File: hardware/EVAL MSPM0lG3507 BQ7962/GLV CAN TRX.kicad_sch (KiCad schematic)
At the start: 29 parts, among them U10 MCP2542FDxMF, U11 FCX495, U8 FCX495, U9 LMR51603XDBVR

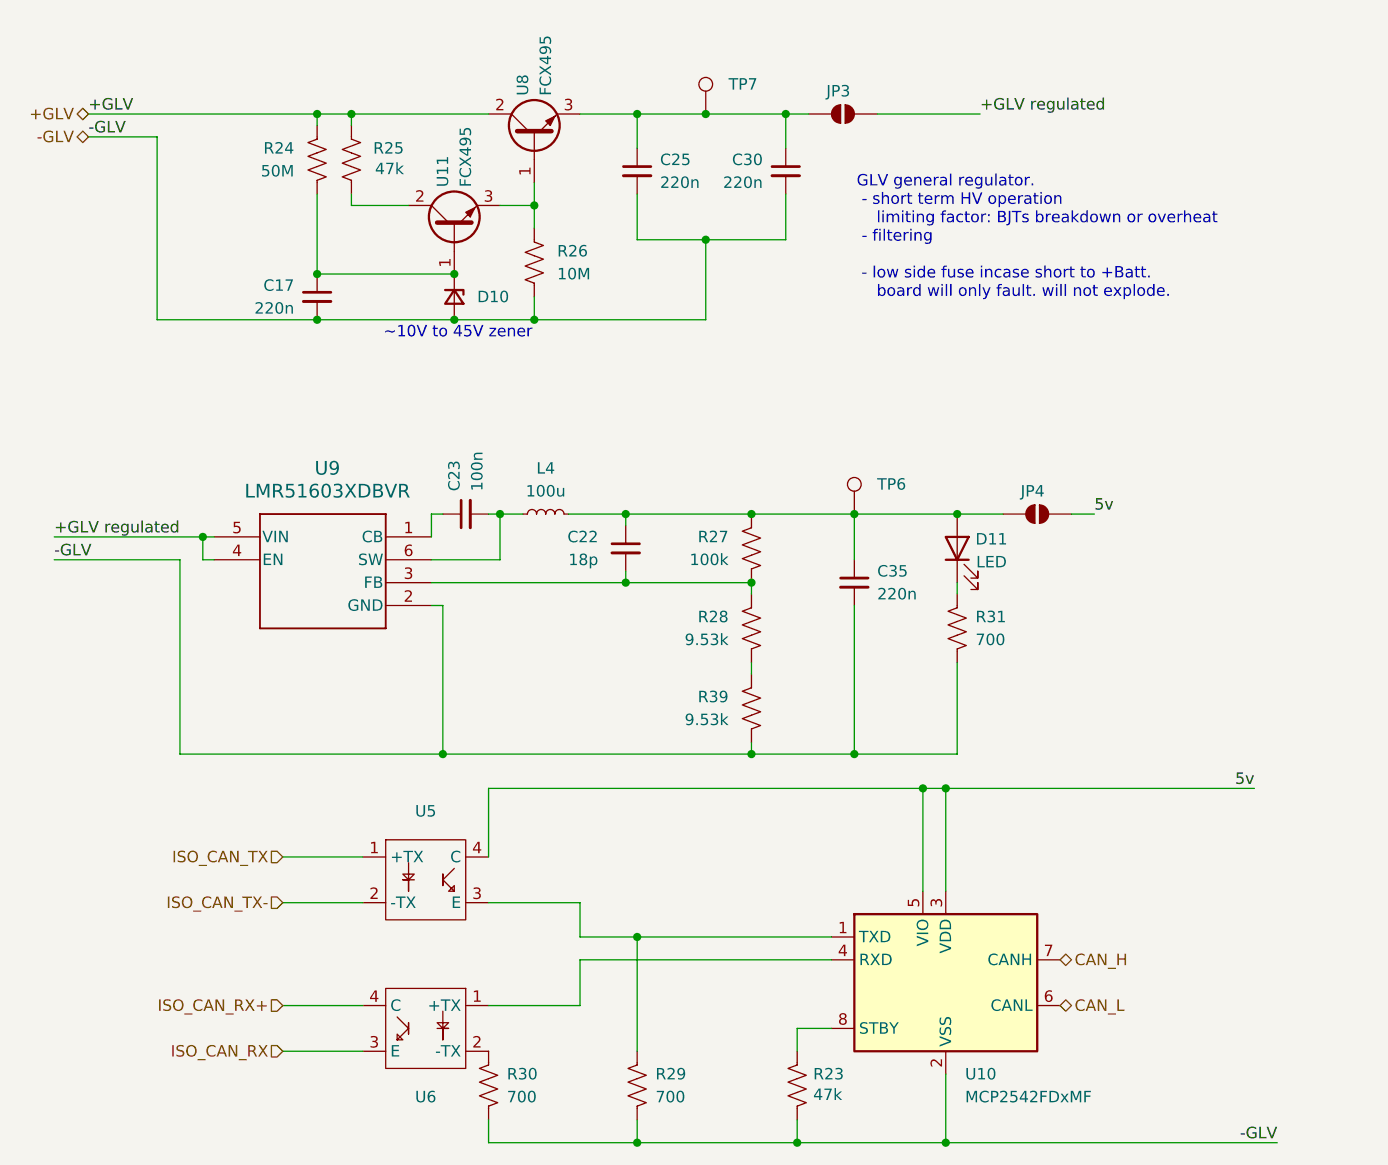
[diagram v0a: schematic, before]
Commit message: cleaned up schematics
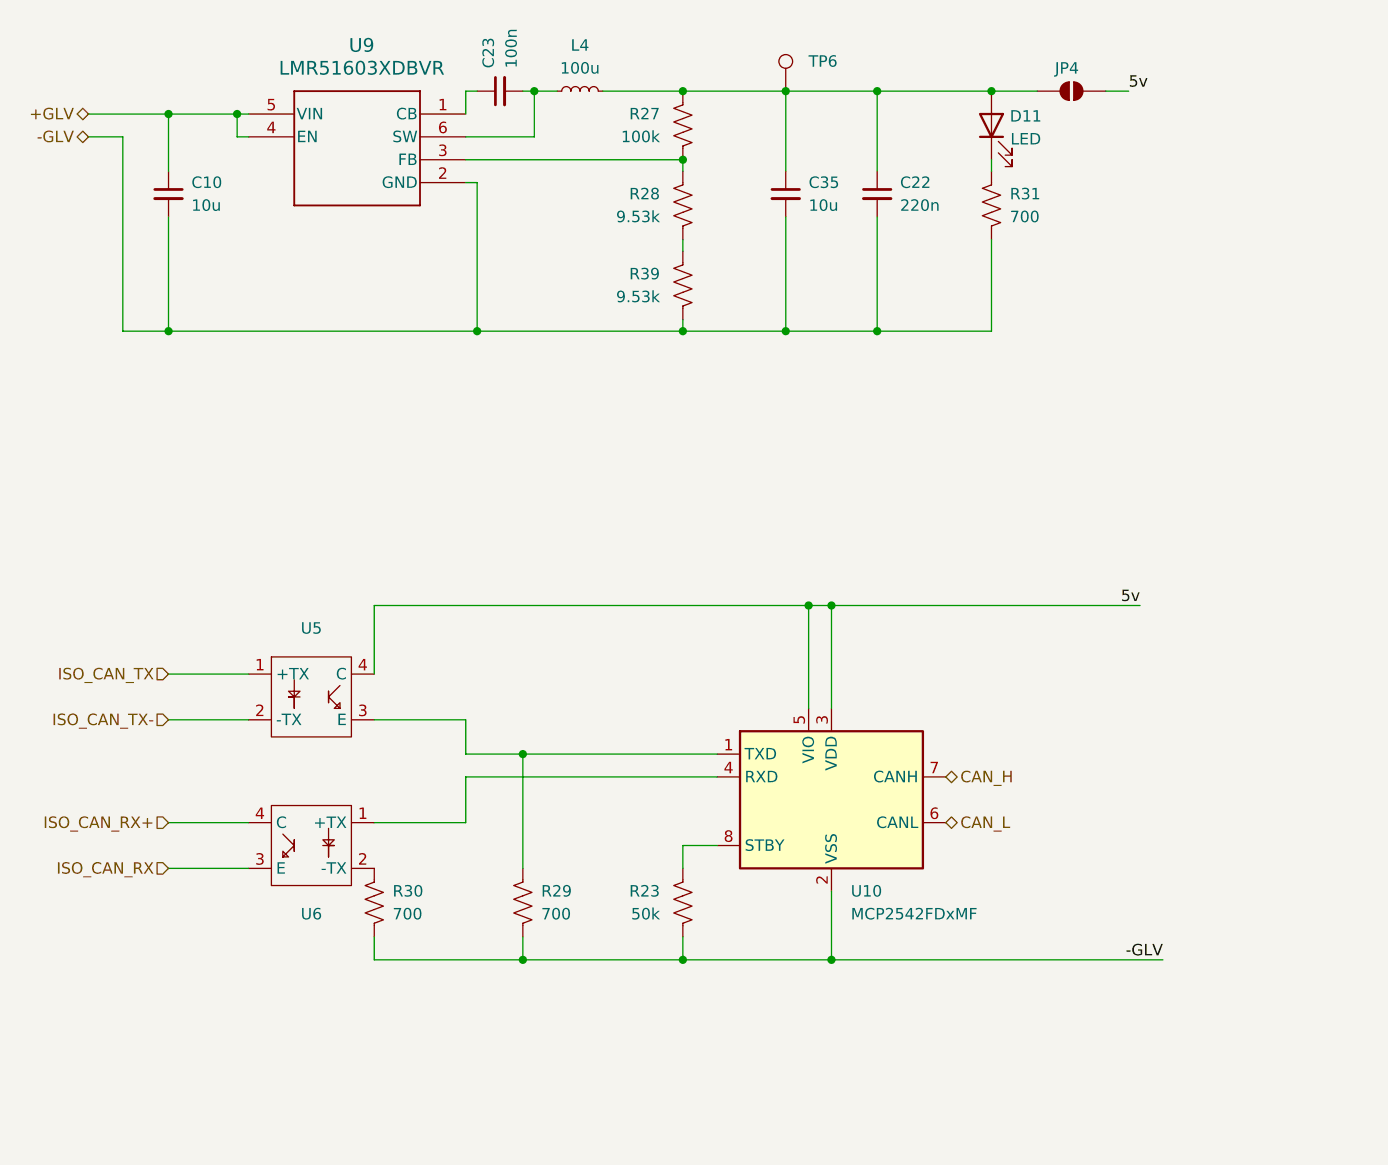
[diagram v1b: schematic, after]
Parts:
- removed C17, C25, C30: 220n, Capacitor_SMD:C_1206_3216Metric_Pad1.33x1.80mm_HandSolder, symbol Device:C_Small
- removed D10: 36V, Diode_SMD:D_SOD-123, symbol Device:D_Zener_Small
- removed JP3: SolderJumper_2_Open, Jumper:SolderJumper-2_P1.3mm_Open_TrianglePad1.0x1.5mm, symbol Jumper:SolderJumper_2_Open
- removed R24: 50M, Resistor_SMD:R_1206_3216Metric_Pad1.30x1.75mm_HandSolder, symbol Device:R_US
- removed R25: 47k, Resistor_SMD:R_1206_3216Metric_Pad1.30x1.75mm_HandSolder, symbol Device:R_US
- removed R26: 10M, Resistor_SMD:R_1206_3216Metric_Pad1.30x1.75mm_HandSolder, symbol Device:R_US
- removed TP7: TestPoint, TestPoint:TestPoint_Loop_D2.50mm_Drill1.0mm_LowProfile, symbol Connector:TestPoint
- removed U11, U8: FCX495, Package_TO_SOT_SMD:SOT-89-3, symbol zzLocalLibrary:FCX485_NPN_BJT
- added C10: 10u, Capacitor_SMD:C_1206_3216Metric_Pad1.33x1.80mm_HandSolder, symbol Device:C_Small
- C22: value 18p -> 220n
- C35: value 220n -> 10u; mouser (none) -> https://www.mouser.com/ProductDetail/Samsung-Electro-Mechan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
- D11: footprint LED_SMD:LED_0805_2012Metric_Pad1.15x1.40mm_HandSolder -> LED_SMD:LED_0201_0603Metric_Pad0.64x0.40mm_HandSolder; mouser (none) -> https://www.mouser.com/ProductDetail/Inolux/IN-S63AT5A?qs=s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
- R23: value 47k -> 50k; mouser (none) -> https://www.mouser.com/ProductDetail/YAGEO/RT1206BRD0750KL?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
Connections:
- net +GLV regulated is gone; now on net +GLV: U9.4 (EN), U9.5 (VIN)
- net +GLV: now also C10.1
- net -GLV: now also C22.2, R23.1, C10.2; no longer R23.2
- net at R27.1, R28.2, U9.3 (FB): no longer C22.2
- net at U10.8 (STBY): now also R23.2; no longer R23.1
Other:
- note removed: "GLV general regulator. - short term HV operation limiting factor: BJTs breakdown or overheat - filtering - low side fuse incase short to +Batt. board will only fault. will not explode."
- note removed: "~10V to 45V zener"
- moved on the sheet: C23, C35, D11, JP4, L4, R27, R28, R29, R30, R31, R39, TP6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
